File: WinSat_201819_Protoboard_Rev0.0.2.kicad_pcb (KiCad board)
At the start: 4 copper layers, 35.5 x 57.5 mm, 73 parts, among them J1 Conn_01x02_Female, J10 Conn_01x06_Male, J11 USB_B_Micro, J2 Conn_01x02_Female, J3 Conn_01x02_Female, J4 Conn_01x02_Female, J5 Conn_01x03_Female, J6 Conn_01x02_Female, J7 JTAG-6PIN, J8 Conn_01x03_Female, J9 Conn_01x03_Female, P1 TPS82150, Q1 SSM3K329R, Q2 SSM3K329R, Q3 SSM3K329R, Q4 Package_TO_SOT_SMD:SOT-23, U1 LTC4361, U10 XBEE_PRO900, U2 Si1470DH, U3 BMP280, U9 ATxmega128A4-AU

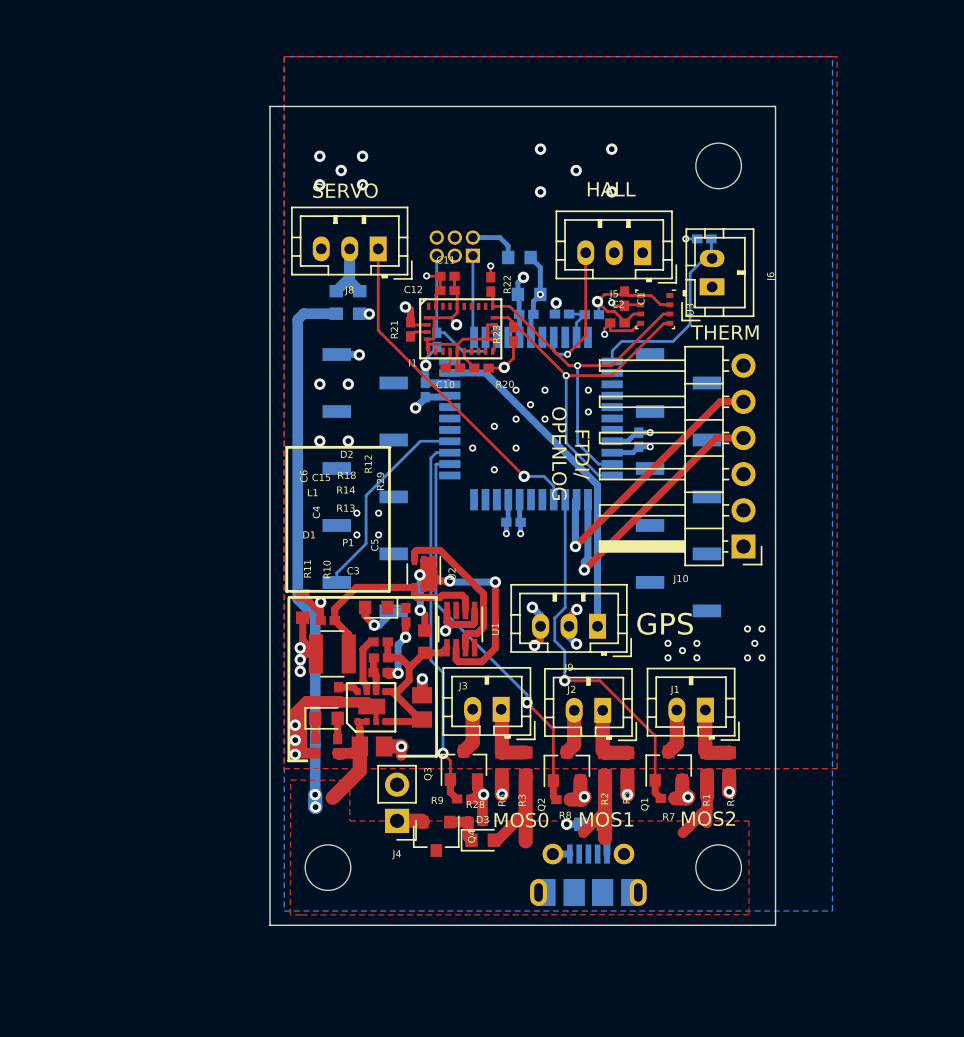
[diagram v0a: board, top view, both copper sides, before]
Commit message: Fixed Issues Thomas Saw
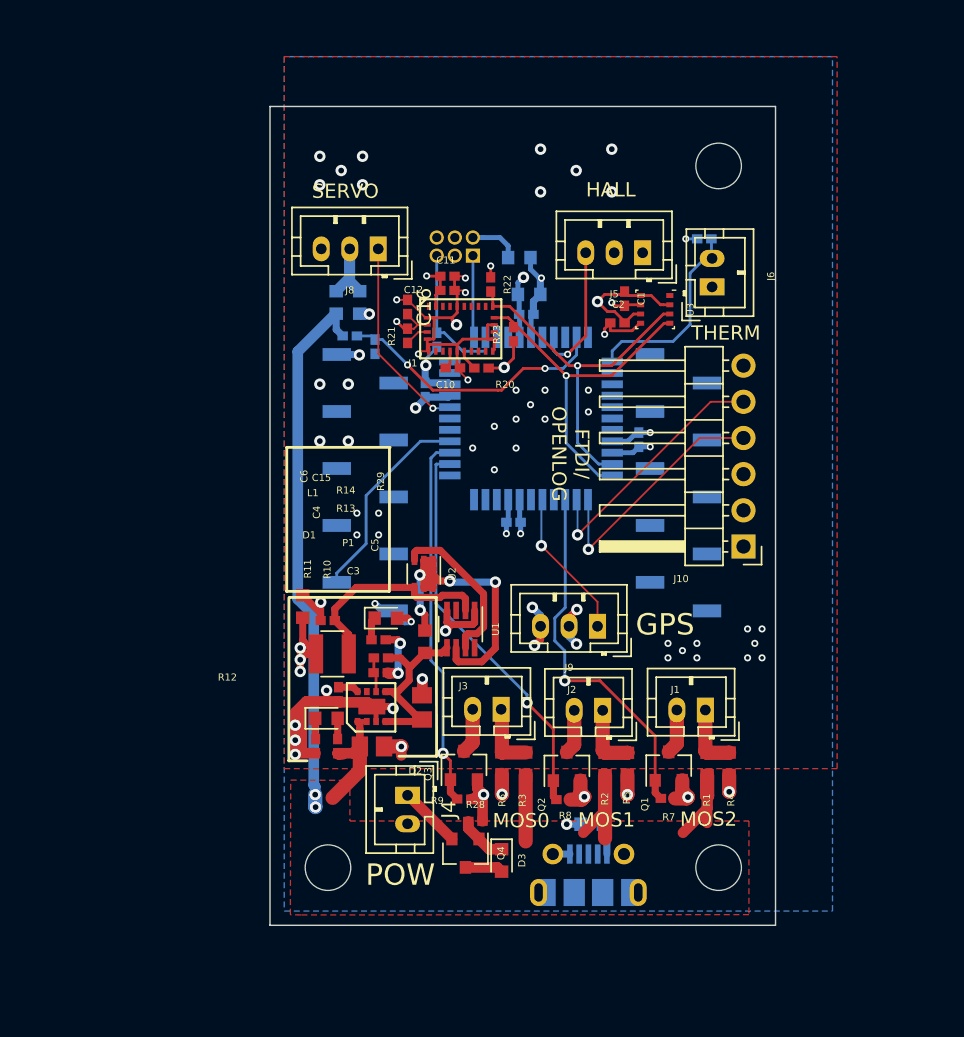
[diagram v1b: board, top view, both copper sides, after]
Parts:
- removed R18: 100k, OSD335x-KiCad-master:Not_Broken_0402
- added C16: 100nF, OSD335x-KiCad-master:Not_Broken_0402, F.Cu at (73.7, 84.6)
- J4: footprint Connector_PinHeader_2.54mm:PinHeader_1x02_P2.54mm_Vertical -> Connector_JST:JST_PH_B2B-PH-K_1x02_P2.00mm_Vertical
- R25: value 66K -> 7.15K
- moved R24 17.1 mm to (69.6, 86.6), turned to 180 degrees
- moved R25 13.3 mm to (71.4, 87.4), turned to 90 degrees
- moved R12 2.58 mm to (71.6, 108.0), turned to 0 degrees
- moved Q4 2.37 mm to (77.7, 122.9)
- moved D3 1.94 mm to (80.3, 123.4), turned to 270 degrees
- moved J4 1.94 mm to (73.7, 118.9), turned to 270 degrees
- moved D2 1.01 mm to (72.1, 106.4), turned to 0 degrees
- moved R21 0.50 mm to (73.7, 86.6)
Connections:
- R24 pad 2: +3V3 -> BAT_POS
- U9 pad 15: SERVO_TCL -> Net-(U9-Pad15)
- U9 pad 16: Net-(U9-Pad16) -> GPS_TX-MCU_RX
- U9 pad 29: Net-(U9-Pad29) -> SERVO_TCL
- U9 pad 32: GPS_TX-MCU_RX -> Net-(U9-Pad32)
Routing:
- net VOLTDIV_ADC: track 2.93 -> 19.3 mm, vias 0 -> 2
- net GPS_TX-MCU_RX: track 23.5 -> 10.6 mm, vias 0 -> 1
- net SERVO_TCL: track 23.5 -> 14.0 mm
- net GND: track 91.4 -> 99.6 mm, vias 63 -> 69
- net Net-(P1-Pad7): track 4.05 -> 0.00 mm
- net Net-(J4-Pad1): track 1.84 -> 4.38 mm
- net FTDI_OLOG_TX-MCU_RX: track 20.1 -> 17.6 mm
- net +3V3: track 51.9 -> 53.6 mm, vias 18 -> 19
- net FTDI_OLOG_RX-MCU_TX: track 19.3 -> 18.0 mm
- net REG_OUT: track 14.6 -> 13.4 mm
- net Net-(D3-Pad1): track 2.74 -> 3.43 mm
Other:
- board text added: "POW"

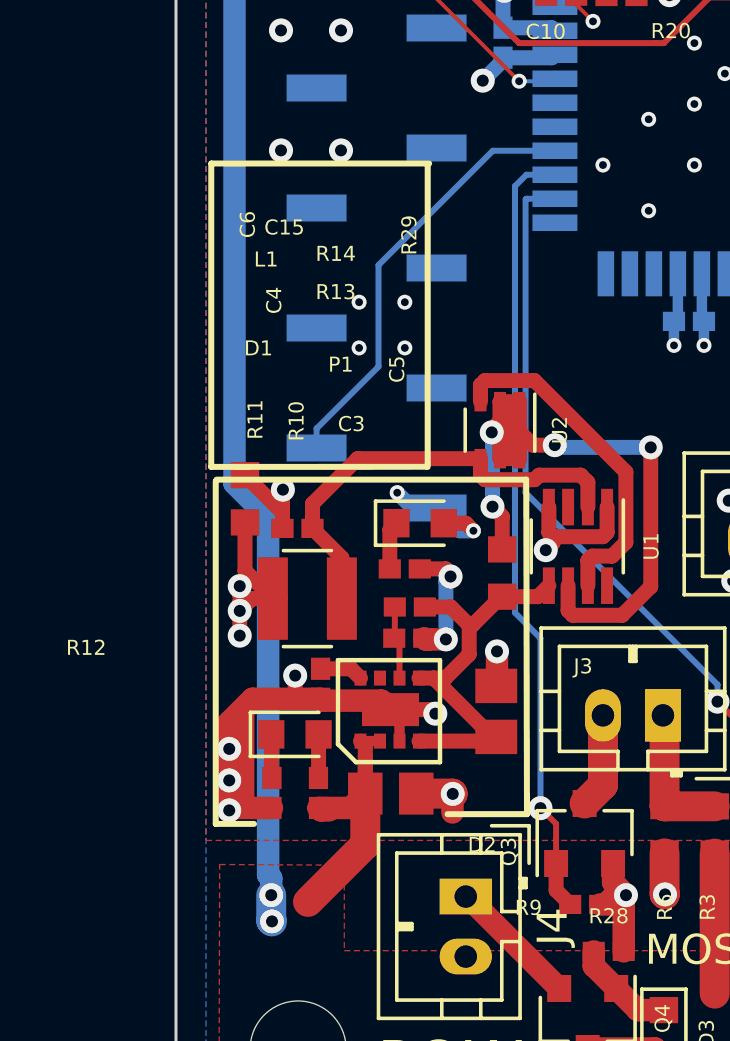
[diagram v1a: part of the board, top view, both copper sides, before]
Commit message: Not sure what updated.
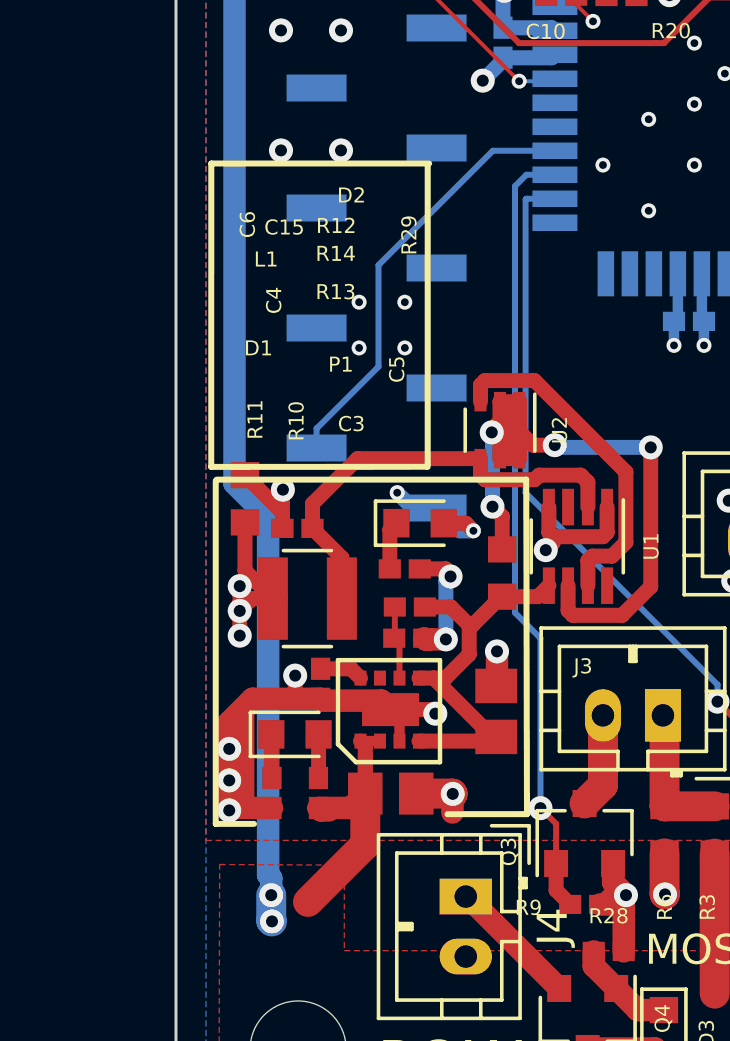
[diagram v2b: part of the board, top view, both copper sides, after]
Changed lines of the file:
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@@
     (tags resistor)
     (attr smd)
-    (fp_text reference R12 (at -10.6194 2.6332) (layer F.SilkS)
+    (fp_text reference R12 (at -2.286 -11.43) (layer F.SilkS)
       (effects (font (size 0.5 0.5) (thickness 0.08)))
     )
@@
     (tags diode)
     (attr smd)
-    (fp_text reference D2 (at 2.0697 10.7298) (layer F.SilkS)
-      (effects (font (size 0.5 0.5) (thickness 0.08)))
-    )
+    (fp_text reference D2 (at -2.286 -10.922) (layer F.SilkS)
+      (effects (font (size 0.5 0.5) (thickness 0.08)))
+    )

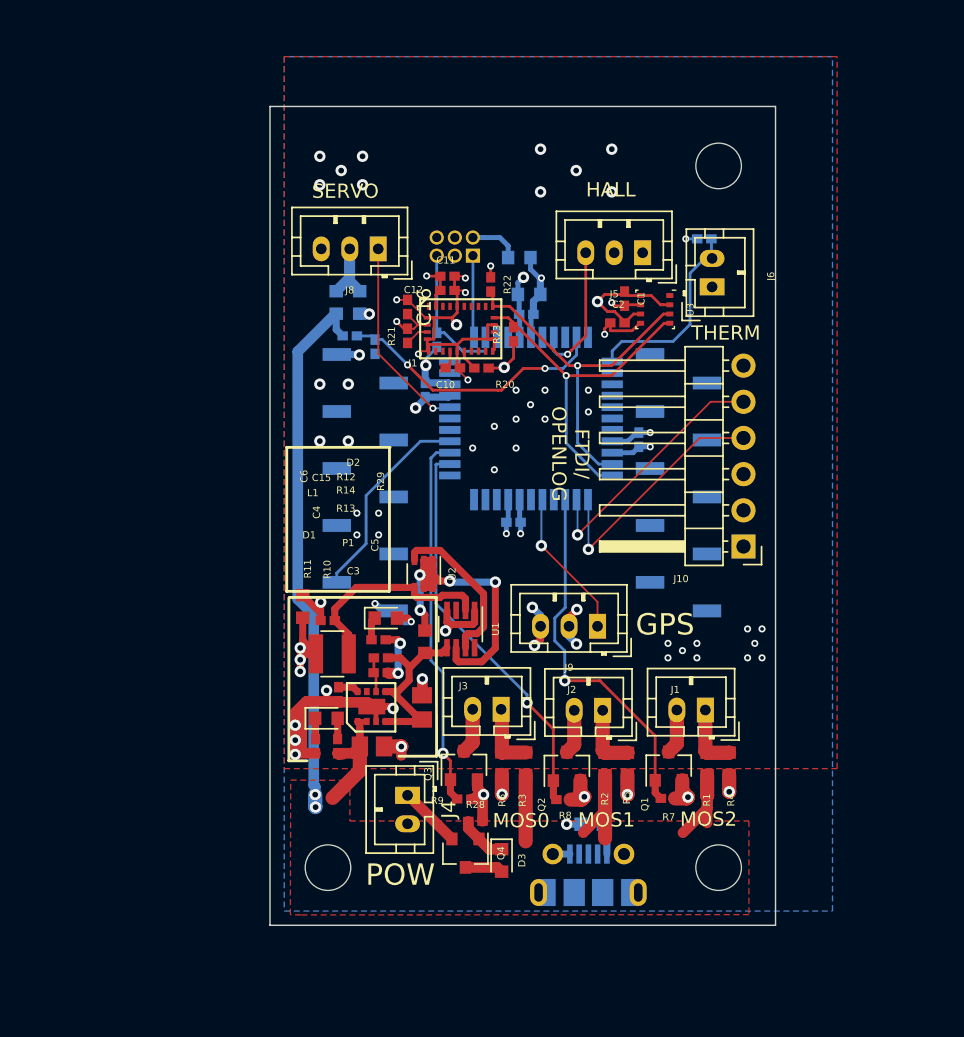
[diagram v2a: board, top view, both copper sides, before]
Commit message: Change Board Size
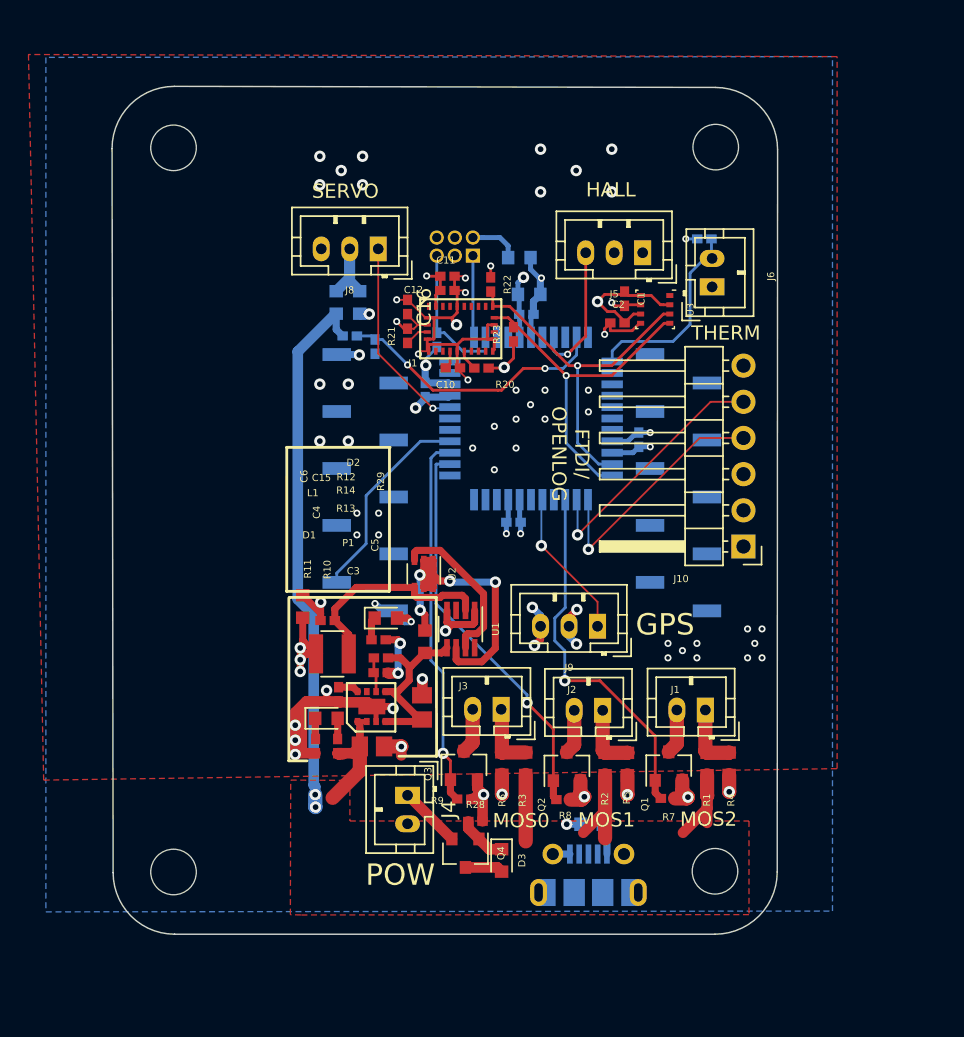
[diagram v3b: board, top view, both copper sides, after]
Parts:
- added MK4: Mounting_Hole, MountingHole:MountingHole_3.2mm_M3, F.Cu at (57.2, 73.4)
- R29: value 0.025 OHM -> 0.05 OHM
- moved MK3 10.9 mm to (57.2, 124.3)
- moved MK2 1.34 mm to (95.3, 73.4)
- moved MK1 0.36 mm to (95.2, 124.2)
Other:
- board size 35.5 x 57.5 mm -> 46.7 x 59.5 mm
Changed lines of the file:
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@@
   (general
     (thickness 1.6)
-    (drawings 23)
+    (drawings 27)
     (tracks 616)
     (zones 0)
-    (modules 73)
+    (modules 74)
     (nets 102)
   )
@@
   (layers
     (0 F.Cu mixed)
-    (1 In1.Cu power)
-    (2 In2.Cu power)
+    (1 In1.Cu power hide)
+    (2 In2.Cu power hide)
     (31 B.Cu jumper)
     (36 B.SilkS user)
     (37 F.SilkS user)
-    (38 B.Mask user)
+    (38 B.Mask user hide)
     (39 F.Mask user)
     (44 Edge.Cuts user)
-    (45 Margin user)
+    (45 Margin user hide)
     (46 B.CrtYd user)
     (47 F.CrtYd user)
@@
     (add_net XBEE_TX-MCU_RX)
   )
+  (module MountingHole:MountingHole_3.2mm_M3 (layer F.Cu)
+    (at 57.2262 73.406)
+    (descr "Mounting Hole 3.2mm, no annular, M3")
+    (tags "mounting hole 3.2mm no annular m3")
+    (attr virtual)
+    (fp_text reference MK4 (at 0 -4.2) (layer F.SilkS) hide
+      (effects (font (size 1 1) (thickness 0.15)))
+    )
+    (fp_text value Mounting_Hole (at 0 4.2) (layer F.Fab)
+      (effects (font (size 1 1) (thickness 0.15)))
+    )
+    (fp_text user %R (at 0.3 0) (layer F.Fab)
+      (effects (font (size 1 1) (thickness 0.15)))
+    )
+    (fp_circle (center 0 0) (end 3.2 0) (layer Cmts.User) (width 0.15))
+    (fp_circle (center 0 0) (end 3.45 0) (layer F.CrtYd) (width 0.05))
+    (pad 1 np_thru_hole circle (at 0 0) (size 3.2 3.2) (drill 3.2) (layers *.Cu *.Mask))
+  )
   (module OSD335x-KiCad-master:Not_Broken_0402 (layer F.Cu)
     (at 73.66 84.582 270)
@@
   )
   (module MountingHole:MountingHole_3.2mm_M3 (layer F.Cu)
-    (at 95.504 123.952)
+    (at 95.25 124.206)
     (descr "Mounting Hole 3.2mm, no annular, M3")
     (tags "mounting hole 3.2mm no annular m3")
@@
   )
   (module MountingHole:MountingHole_3.2mm_M3 (layer F.Cu)
-    (at 95.504 74.676)
+    (at 95.3008 73.3552)
     (descr "Mounting Hole 3.2mm, no annular, M3")
     (tags "mounting hole 3.2mm no annular m3")
@@
   )
   (module MountingHole:MountingHole_3.2mm_M3 (layer F.Cu)
-    (at 68.072 123.952)
+    (at 57.2262 124.2568)
     (descr "Mounting Hole 3.2mm, no annular, M3")
     (tags "mounting hole 3.2mm no annular m3")
@@
       (effects (font (size 0.5 0.5) (thickness 0.08)))
     )
-    (fp_text value "0.025 OHM" (at 0 1.43 90) (layer F.Fab)
+    (fp_text value "0.05 OHM" (at 0 1.43 90) (layer F.Fab)
       (effects (font (size 1 1) (thickness 0.15)))
     )
@@
     )
   )
+  (gr_line (start 95.2754 69.1642) (end 57.277 69.088) (layer Edge.Cuts) (width 0.1))
+  (gr_line (start 99.6188 124.2568) (end 99.6442 73.533) (layer Edge.Cuts) (width 0.1))
+  (gr_line (start 57.3024 128.6256) (end 95.25 128.6256) (layer Edge.Cuts) (width 0.1))
+  (gr_line (start 52.9082 73.4568) (end 52.9844 124.3076) (layer Edge.Cuts) (width 0.1))
+  (gr_arc (start 95.2754 73.533) (end 99.6442 73.533) (angle -90) (layer Edge.Cuts) (width 0.1))
+  (gr_arc (start 95.25 124.2568) (end 95.25 128.6256) (angle -90) (layer Edge.Cuts) (width 0.1))
+  (gr_arc (start 57.3024 124.3076) (end 52.9844 124.3076) (angle -90) (layer Edge.Cuts) (width 0.1))
+  (gr_arc (start 57.277 73.4568) (end 57.277 69.088) (angle -90) (layer Edge.Cuts) (width 0.1))
   (gr_text POW (at 73.152 124.46) (layer F.SilkS)
     (effects (font (size 1.5 1.5) (thickness 0.3)))
@@
     (effects (font (size 1 1) (thickness 0.25)))
   )
-  (gr_line (start 99.5 70.5) (end 64 70.5) (layer Edge.Cuts) (width 0.1))
-  (gr_line (start 99.5 128) (end 99.5 70.5) (layer Edge.Cuts) (width 0.1))
-  (gr_line (start 64 128) (end 99.5 128) (layer Edge.Cuts) (width 0.1))
-  (gr_line (start 64 70.5) (end 64 128) (layer Edge.Cuts) (width 0.1))
   (gr_line (start 75.7 116.125) (end 73.05 116.125) (layer F.SilkS) (width 0.2))
   (gr_line (start 75.675 104.975) (end 75.7 116.125) (layer F.SilkS) (width 0.2))
@@
     (polygon
       (pts
-        (xy 65 127) (xy 103.825 127.175) (xy 104 67) (xy 65.175 66.825)
+        (xy 48.6946 127.0278) (xy 103.825 127.175) (xy 104 67) (xy 48.8696 66.8528)
       )
     )
@@
     (polygon
       (pts
-        (xy 65 127) (xy 103.5 127) (xy 103.5 67) (xy 65 67)
+        (xy 48.768 126.9036) (xy 103.5 127) (xy 103.5 67) (xy 48.768 66.9036)
       )
     )
@@
     (polygon
       (pts
-        (xy 65 67) (xy 65 117) (xy 103.825 117) (xy 103.825 67)
+        (xy 47.0408 66.8528) (xy 48.1076 117.8052) (xy 103.825 117) (xy 103.825 67)
       )
     )
@@
     (polygon
       (pts
-        (xy 65 67) (xy 65 127) (xy 103.5 127) (xy 103.5 67)
+        (xy 48.26 67.056) (xy 48.26 127.056) (xy 103.5 127) (xy 103.5 67)
       )
     )
